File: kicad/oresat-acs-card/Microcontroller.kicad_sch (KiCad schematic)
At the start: 23 parts, among them J2 ORESAT-DEBUG-CONNECTOR-SOLAR, U14 TCAN330GDCNT, U15 STM32F042K6T7, X2 ECS-160-10-36Q-ES-TR

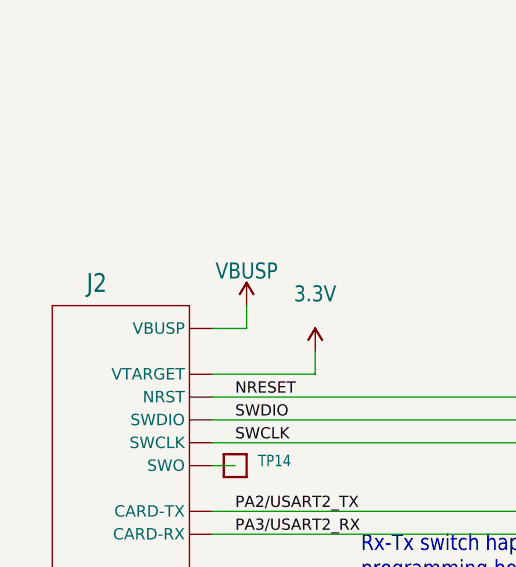
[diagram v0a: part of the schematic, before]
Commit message: Design review changes.
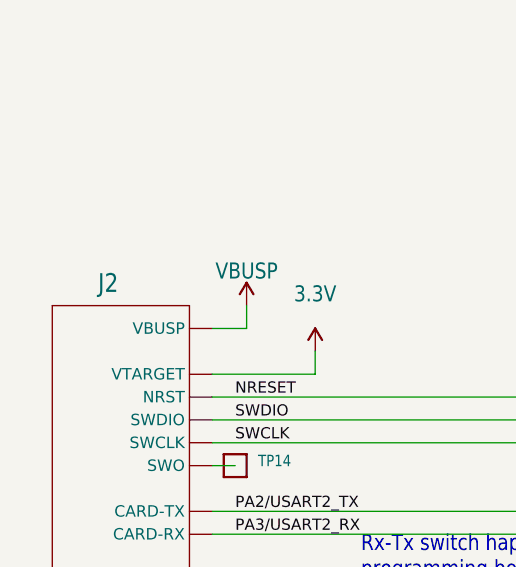
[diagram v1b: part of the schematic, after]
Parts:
- J2: footprint oresat-acs-card:WURTH_687120183622 -> oresat-footprints:J-TE_2-1734592-0; symbol oresat-acs-card-eagle-import:ORESAT-DEBUG-CONNECTOR-SOLAR -> J-TE-2-1734592-0-oresat-debug-connector:J-TE-Debug-2-1734592-0
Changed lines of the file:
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@@
     (pin "1")
   )
-  (symbol (lib_id "oresat-acs-card-eagle-import:ORESAT-DEBUG-CONNECTOR-SOLAR") (at 27.94 198.12 0) (unit 1)
+  (symbol (lib_id "J-TE-2-1734592-0-oresat-debug-connector:J-TE-Debug-2-1734592-0") (at 29.21 198.12 0) (unit 1)
     (in_bom yes) (on_board yes)
-    (property "Reference" "J2" (id 0) (at 25.4 166.37 0)
+    (property "Reference" "J2" (id 0) (at 26.67 166.37 0)
       (effects (font (size 2.0828 1.7703)) (justify left bottom))
     )
-    (property "Value" "ORESAT-DEBUG-CONNECTOR-SOLAR" (id 1) (at 27.94 198.12 0)
+    (property "Value" "ORESAT-DEBUG-CONNECTOR-SOLAR" (id 1) (at 29.21 198.12 0)
       (effects (font (size 1.27 1.27)) hide)
     )
-    (property "Footprint" "oresat-acs-card:WURTH_687120183622" (id 2) (at 27.94 198.12 0)
+    (property "Footprint" "oresat-footprints:J-TE_2-1734592-0" (id 2) (at 29.21 189.23 0)
       (effects (font (size 1.27 1.27)) hide)
     )
-    (property "Datasheet" "" (id 3) (at 27.94 198.12 0)
+    (property "Datasheet" "" (id 3) (at 29.21 189.23 0)
       (effects (font (size 1.27 1.27)) hide)
     )
